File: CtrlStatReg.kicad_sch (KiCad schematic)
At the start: 13 parts, among them Q5 MMBT3904, U18 74LVC74AD, U19 74LVC74AD, U22 74LVC02AD, U24 74LVC125AD, U35 74LVC74AD, U36 74LVC74AD, U37 74LVC74AD

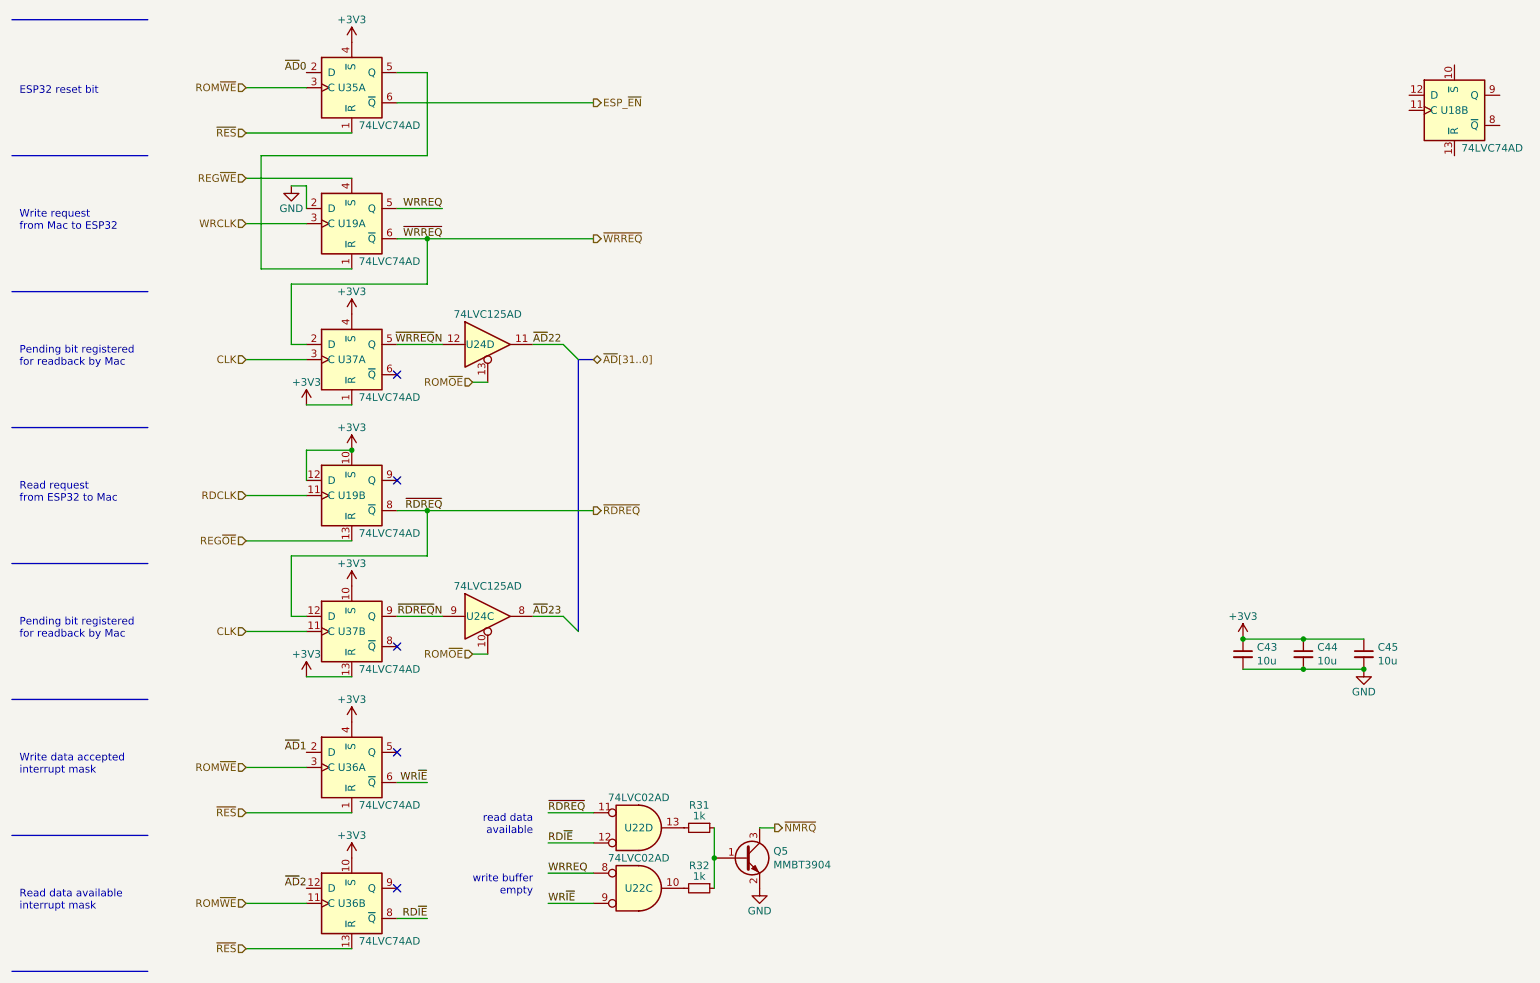
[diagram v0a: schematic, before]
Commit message: Revert "did I mess this up?"
This reverts commit fd75c937204418059e97b488ea791750328fc4dd.
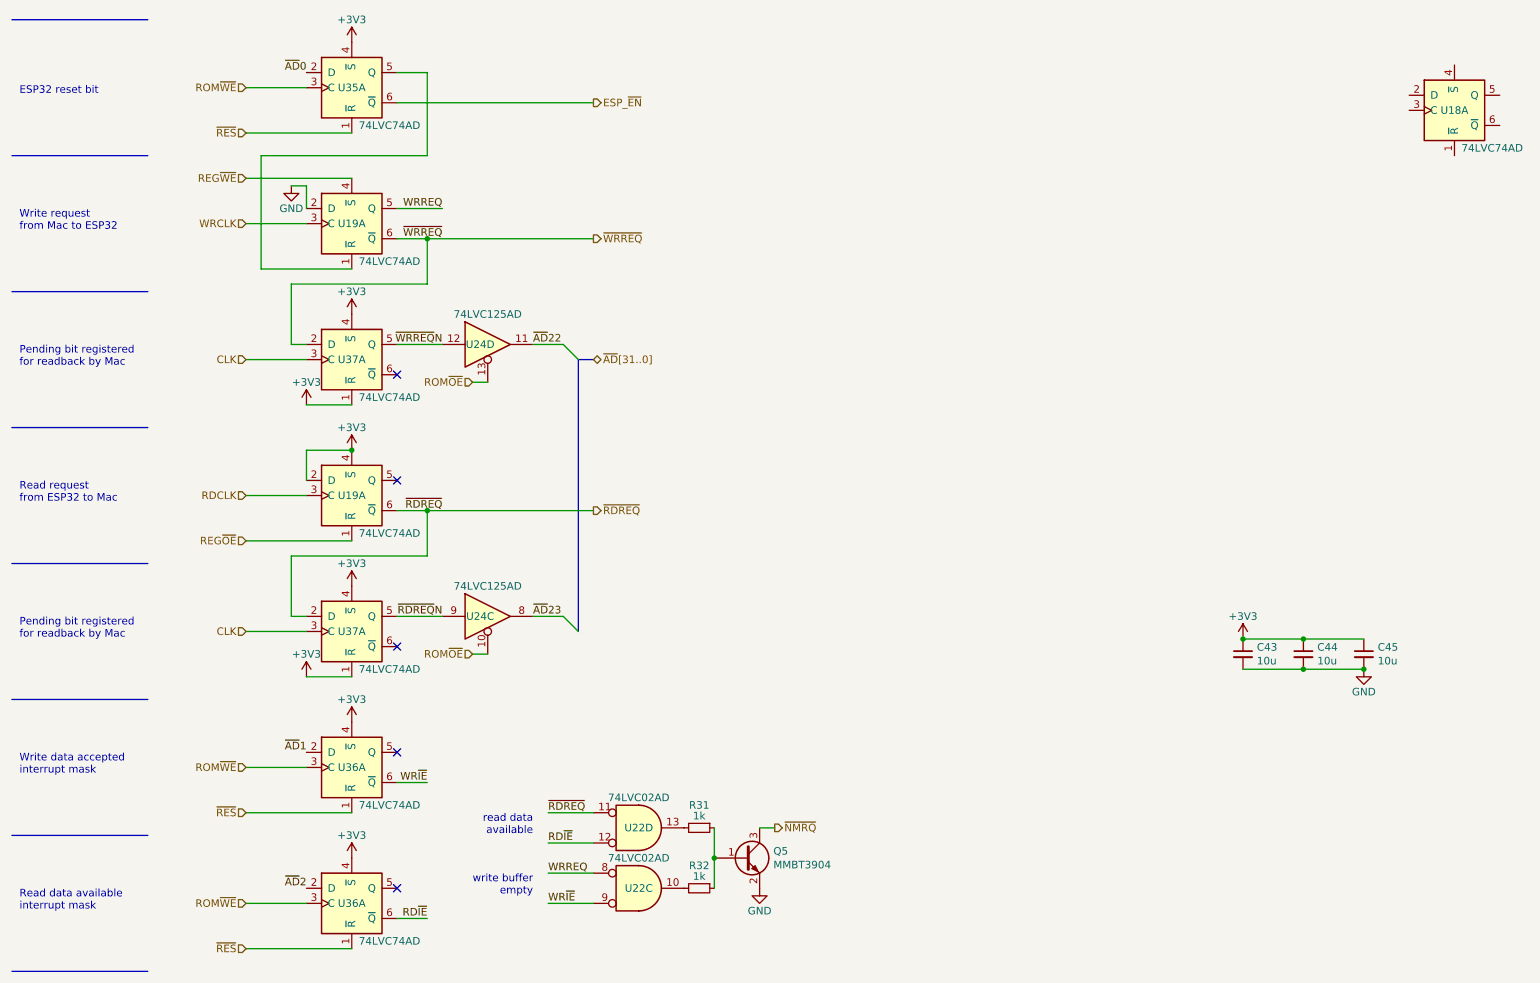
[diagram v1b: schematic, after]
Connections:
- net +3V3: now also U19.2 (D), U19.4 (~{S}), U36.4 (~{S}), U37.1 (~{R}), U37.4 (~{S}); no longer U19.10 (~{S}), U19.12 (D), U36.10 (~{S}), U37.10 (~{S}), U37.13 (~{R})
- net CLK: now also U37.3 (C); no longer U37.11 (C)
- net RDCLK: now also U19.3 (C); no longer U19.11 (C)
- net RD~{IE}: now also U36.6 (~{Q}); no longer U36.8 (~{Q})
- net REG~{OE}: now also U19.1 (~{R}); no longer U19.13 (~{R})
- net ROM~{WE}: now also U36.3 (C); no longer U36.11 (C)
- net ~{AD}2: now also U36.2 (D); no longer U36.12 (D)
- net ~{RDREQ}: now also U19.6 (~{Q}), U37.2 (D); no longer U19.8 (~{Q}), U37.12 (D)
- net ~{RDREQ}N: now also U37.5 (Q); no longer U37.9 (Q)
- net ~{RES}: now also U36.1 (~{R}); no longer U36.13 (~{R})

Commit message: did I mess this up?
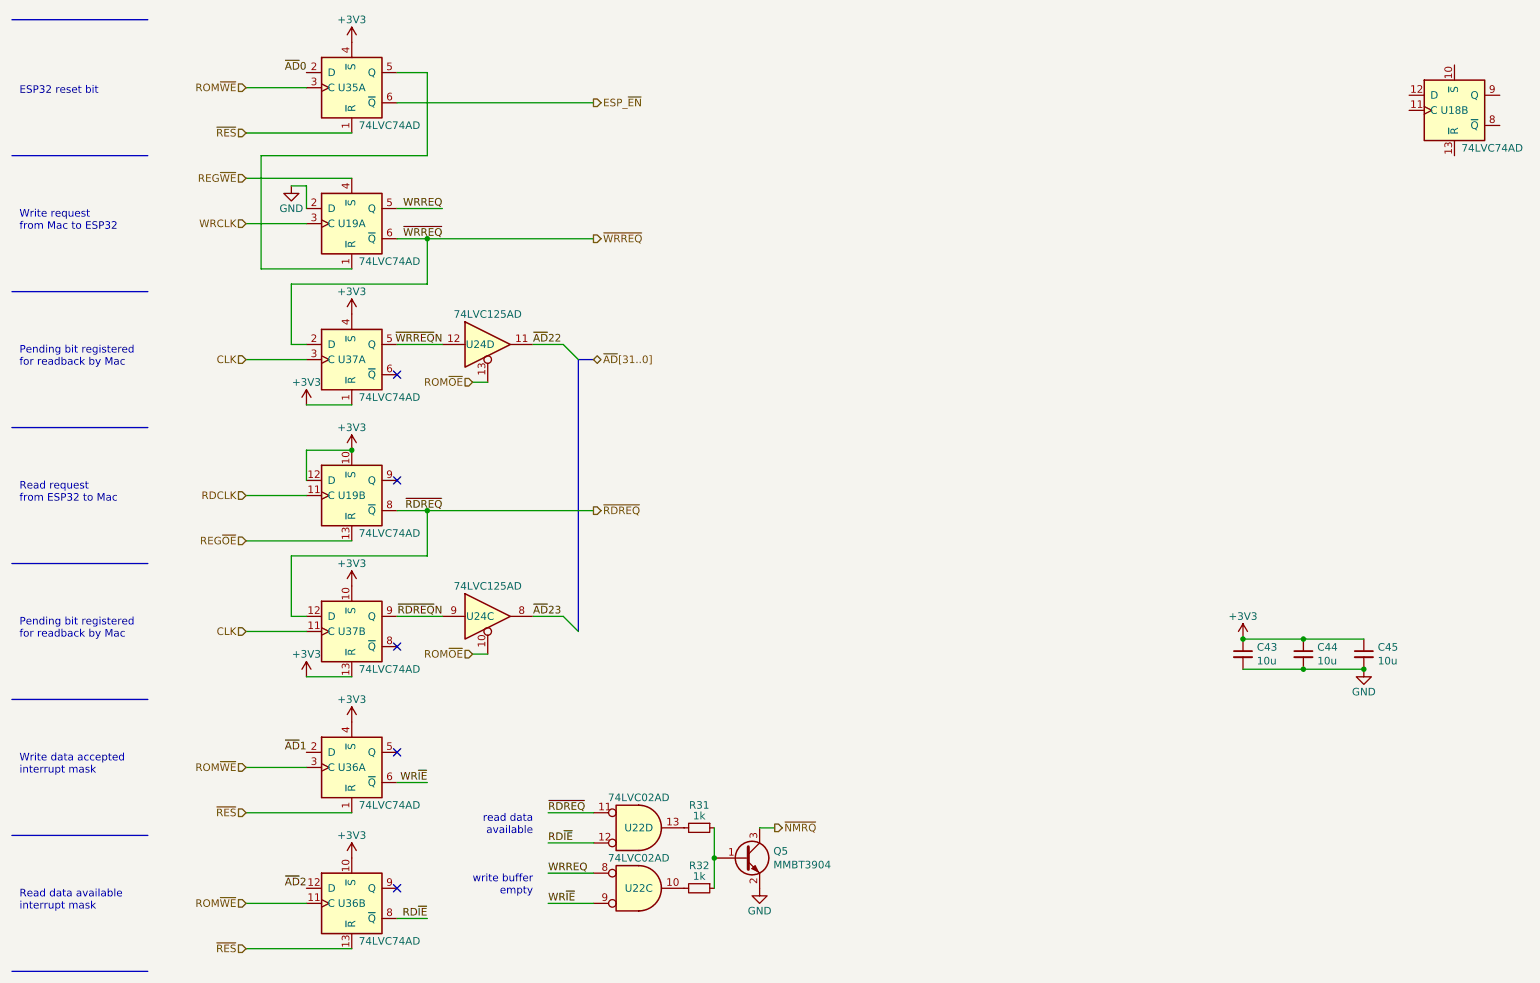
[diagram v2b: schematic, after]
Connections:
- net +3V3: now also U19.10 (~{S}), U19.12 (D), U36.10 (~{S}), U37.10 (~{S}), U37.13 (~{R}); no longer U19.2 (D), U19.4 (~{S}), U36.4 (~{S}), U37.1 (~{R}), U37.4 (~{S})
- net CLK: now also U37.11 (C); no longer U37.3 (C)
- net RDCLK: now also U19.11 (C); no longer U19.3 (C)
- net RD~{IE}: now also U36.8 (~{Q}); no longer U36.6 (~{Q})
- net REG~{OE}: now also U19.13 (~{R}); no longer U19.1 (~{R})
- net ROM~{WE}: now also U36.11 (C); no longer U36.3 (C)
- net ~{AD}2: now also U36.12 (D); no longer U36.2 (D)
- net ~{RDREQ}: now also U19.8 (~{Q}), U37.12 (D); no longer U19.6 (~{Q}), U37.2 (D)
- net ~{RDREQ}N: now also U37.9 (Q); no longer U37.5 (Q)
- net ~{RES}: now also U36.13 (~{R}); no longer U36.1 (~{R})
